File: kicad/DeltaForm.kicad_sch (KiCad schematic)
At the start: 0 parts

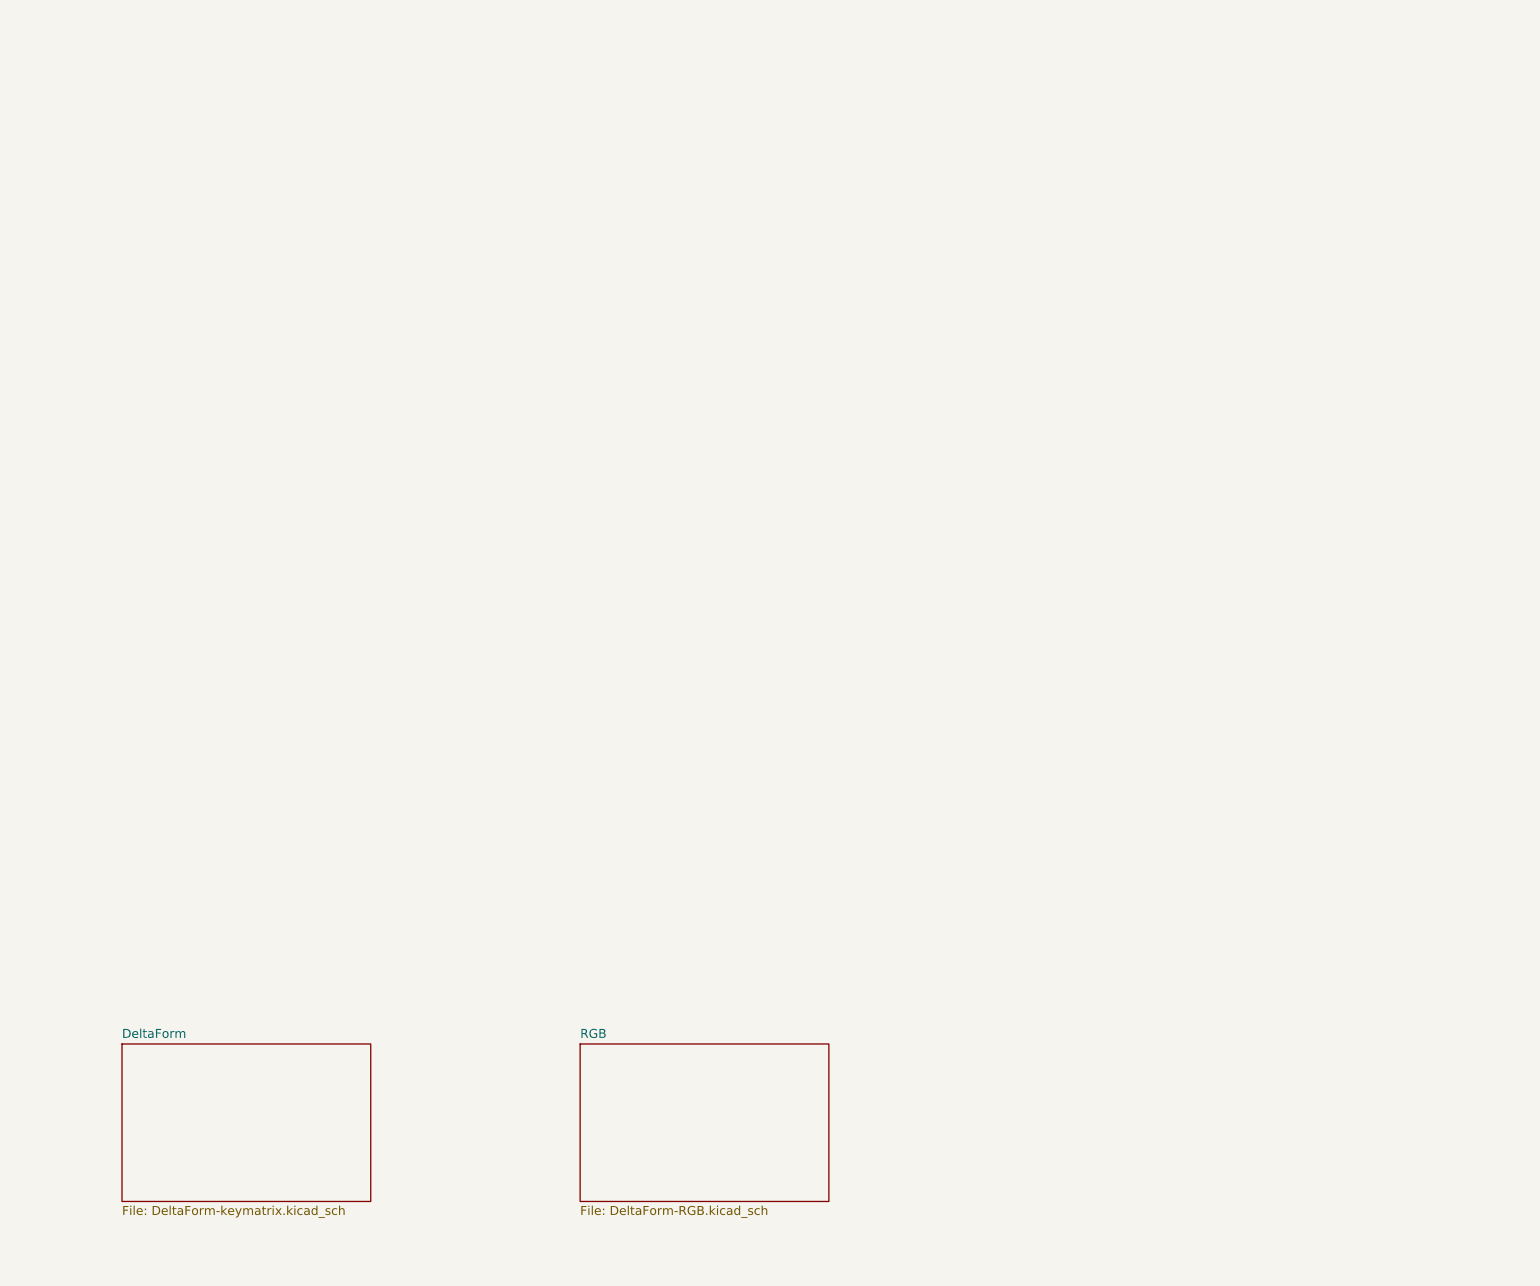
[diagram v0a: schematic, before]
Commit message: reorg schematic (#18)
* GlyphMatrix

* PhaseShift

* DeltaForm
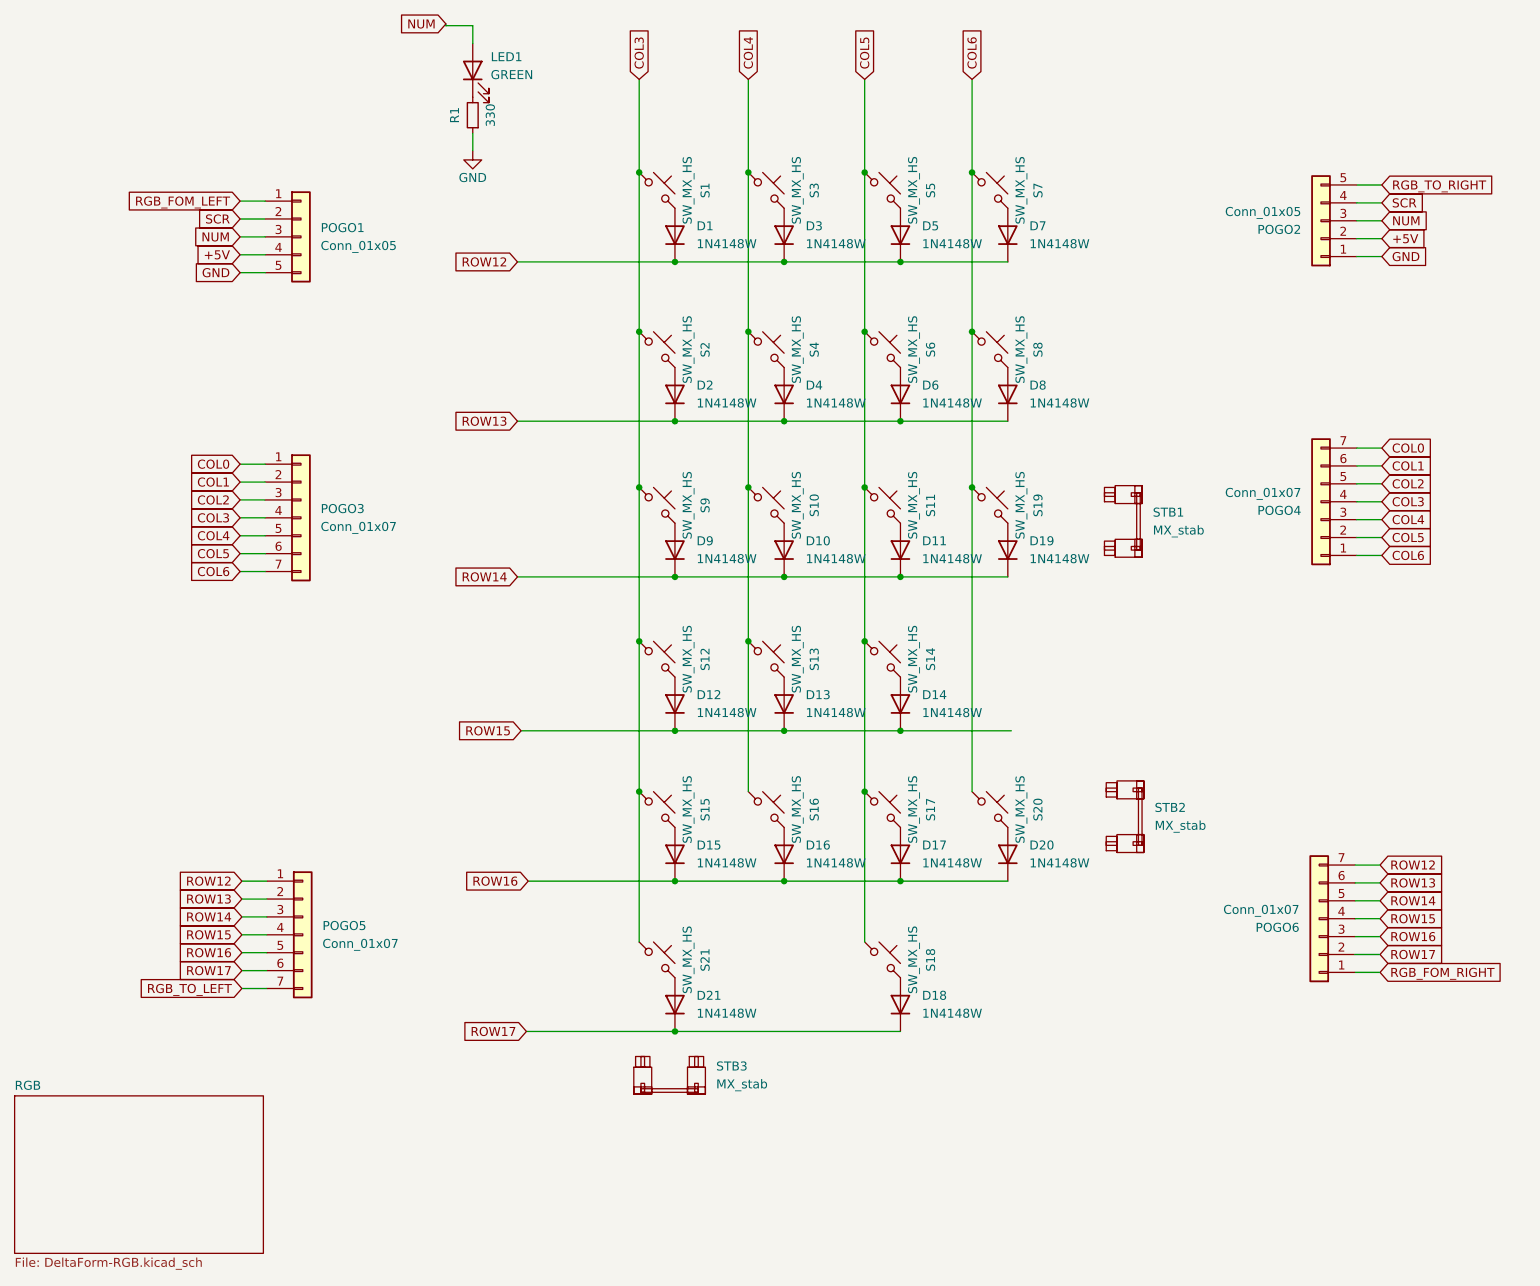
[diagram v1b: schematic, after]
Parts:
- added D1, D10, D11, D12, D13, D14, D15, D16, D17, D18, D19, D2, D20, D21, D3, D4, D5, D6, D7, D8, D9: 1N4148W, TB2086_SMD:D3_SMD, symbol Device:D
- added LED1: GREEN, LED_SMD:LED_0603_1608Metric_Pad1.05x0.95mm_HandSolder, symbol Device:LED
- added POGO1, POGO2: Conn_01x05, TB2086_MISC:Pogopin_1x05_P2.54mm_Curved, symbol Connector_Generic:Conn_01x05
- added POGO3, POGO4, POGO5, POGO6: Conn_01x07, TB2086_MISC:Pogopin_1x07_P2.54mm_Curved, symbol Connector_Generic:Conn_01x07
- added R1: 330, Resistor_SMD:R_0603_1608Metric, symbol Device:R_Small
- added S1, S10, S11, S12, S13, S14, S15, S16, S17, S18, S19, S2, S20, S3, S4, S5, S6, S7, S8, S9: SW_MX_HS, TB2086_KEYSWITCH:SW_MX_HS_1u, symbol TB2086_KEYSWITCH:SW_MX_HS
- added S21: SW_MX_HS, TB2086_KEYSWITCH:SW_MX_HS_2u, symbol TB2086_KEYSWITCH:SW_MX_HS
- added STB1, STB2, STB3: MX_stab, Stabilizer_Cherry_MX_2.00u, symbol PCM_marbastlib-mx:MX_stab
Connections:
- new net: D18.2 (A), S18.1
- new net: D2.2 (A), S2.1
- new net: D12.2 (A), S12.1
- new net: D13.2 (A), S13.1
- new net: D14.2 (A), S14.1
- new net: D1.2 (A), S1.1
- new net: D6.2 (A), S6.1
- new net: D20.2 (A), S20.1
- new net: D19.2 (A), S19.1
- new net: D7.2 (A), S7.1
- new net: D21.2 (A), S21.1
- new net: D3.2 (A), S3.1
- new net: LED1.1 (K), R1.2
- new net: D15.2 (A), S15.1
- new net: D11.2 (A), S11.1
- new net: D10.2 (A), S10.1
- new net: D17.2 (A), S17.1
- new net: D8.2 (A), S8.1
- new net: D16.2 (A), S16.1
- new net: D9.2 (A), S9.1
- new net: D5.2 (A), S5.1
- new net: D4.2 (A), S4.1
- new net +5V: POGO1.4 (Pin_4), POGO2.2 (Pin_2)
- new net COL0: POGO3.1 (Pin_1), POGO4.7 (Pin_7)
- new net COL1: POGO3.2 (Pin_2), POGO4.6 (Pin_6)
- new net COL2: POGO3.3 (Pin_3), POGO4.5 (Pin_5)
- new net COL3: POGO3.4 (Pin_4), POGO4.4 (Pin_4), S1.2, S12.2, S15.2, S2.2, S21.2, S9.2
- new net COL4: POGO3.5 (Pin_5), POGO4.3 (Pin_3), S10.2, S13.2, S16.2, S3.2, S4.2
- new net COL5: POGO3.6 (Pin_6), POGO4.2 (Pin_2), S11.2, S14.2, S17.2, S18.2, S5.2, S6.2
- new net COL6: POGO3.7 (Pin_7), POGO4.1 (Pin_1), S19.2, S20.2, S7.2, S8.2
- new net GND: POGO1.5 (Pin_5), POGO2.1 (Pin_1), R1.1
- new net NUM: LED1.2 (A), POGO1.3 (Pin_3), POGO2.3 (Pin_3)
- new net RGB_FOM_LEFT: POGO1.1 (Pin_1)
- new net RGB_FOM_RIGHT: POGO6.1 (Pin_1)
- new net RGB_TO_LEFT: POGO5.7 (Pin_7)
- new net RGB_TO_RIGHT: POGO2.5 (Pin_5)
- new net ROW12: D1.1 (K), D3.1 (K), D5.1 (K), D7.1 (K), POGO5.1 (Pin_1), POGO6.7 (Pin_7)
- new net ROW13: D2.1 (K), D4.1 (K), D6.1 (K), D8.1 (K), POGO5.2 (Pin_2), POGO6.6 (Pin_6)
- new net ROW14: D10.1 (K), D11.1 (K), D19.1 (K), D9.1 (K), POGO5.3 (Pin_3), POGO6.5 (Pin_5)
- new net ROW15: D12.1 (K), D13.1 (K), D14.1 (K), POGO5.4 (Pin_4), POGO6.4 (Pin_4)
- new net ROW16: D15.1 (K), D16.1 (K), D17.1 (K), D20.1 (K), POGO5.5 (Pin_5), POGO6.3 (Pin_3)
- new net ROW17: D18.1 (K), D21.1 (K), POGO5.6 (Pin_6), POGO6.2 (Pin_2)
- new net SCR: POGO1.2 (Pin_2), POGO2.4 (Pin_4)
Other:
- removed sheet DeltaForm
